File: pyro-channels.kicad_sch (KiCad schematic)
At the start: 22 parts, among them J2 Pyro Channels, J3 Screw Switches, Q2 AO3400A, Q3 AO3400A, Q5 AO3400A, Q6 AO3400A, Q7 AO3400A, Q8 AO3400A

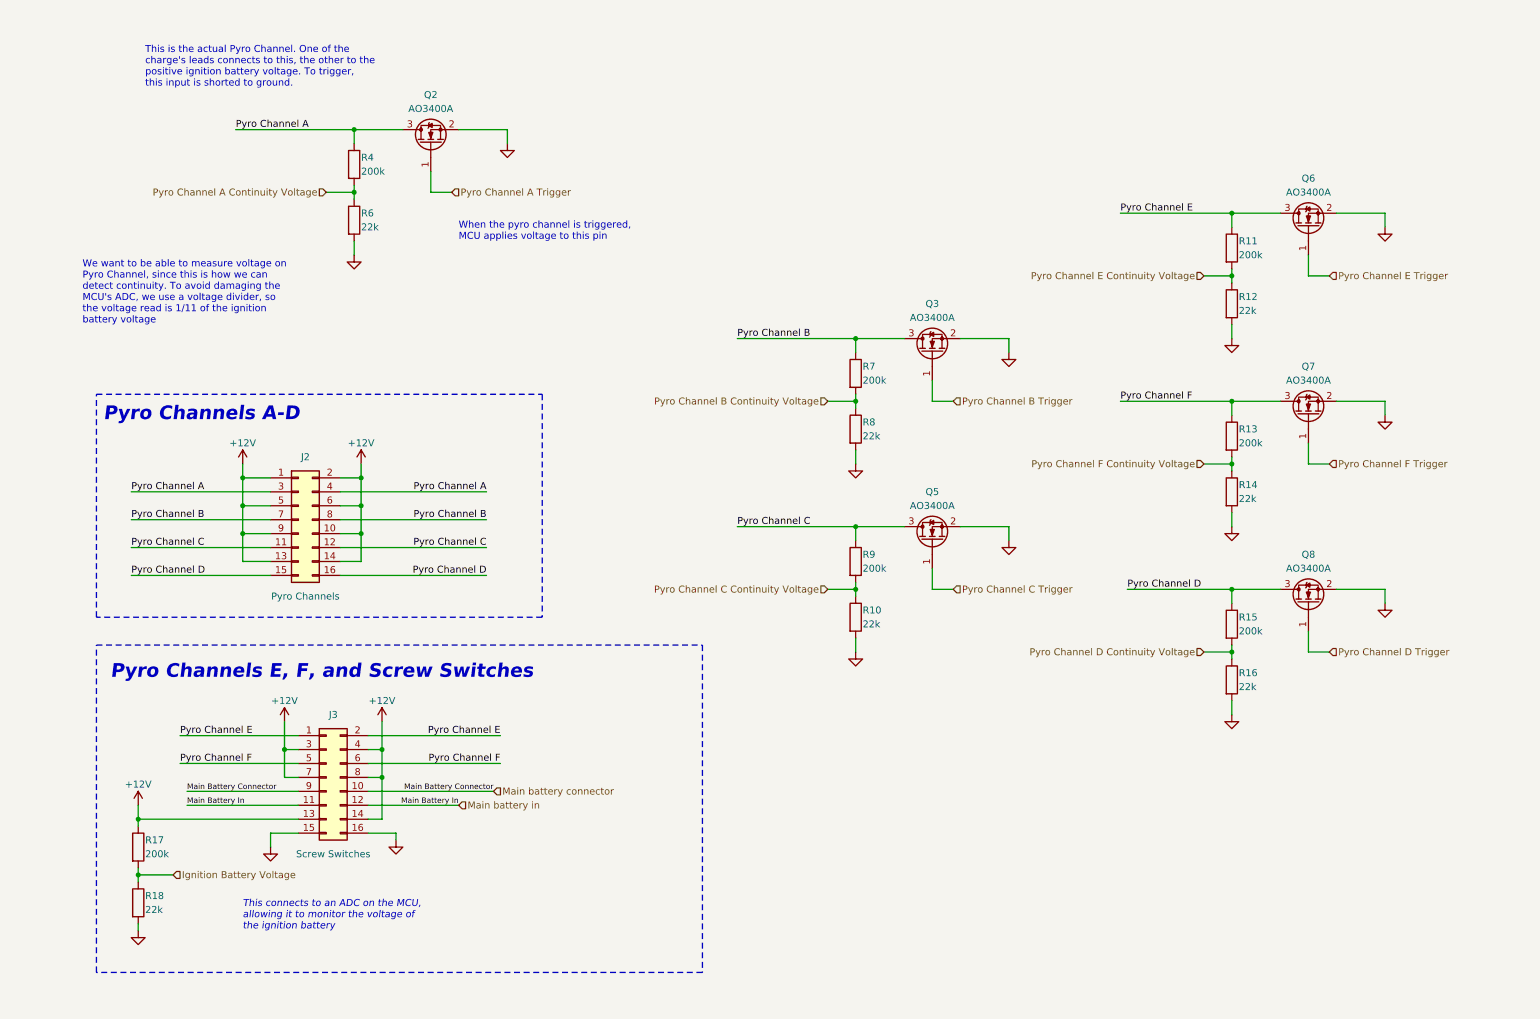
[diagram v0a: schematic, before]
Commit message: Finished updating the schematics
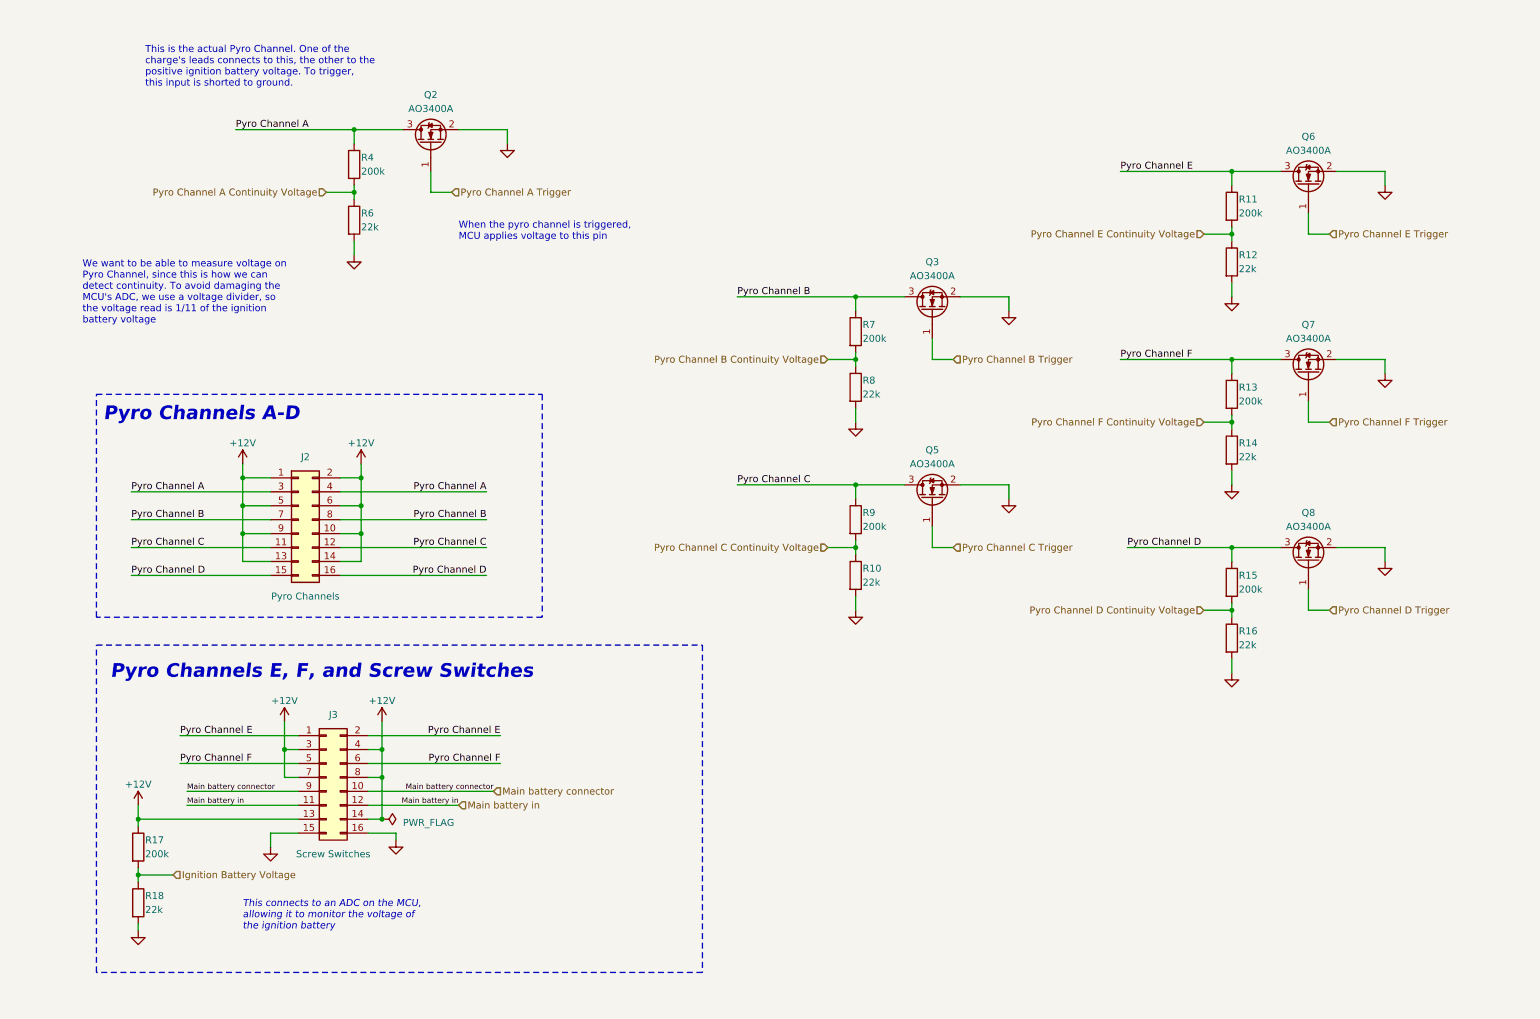
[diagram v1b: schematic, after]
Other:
- moved on the sheet: Q3, Q5, Q6, Q7, Q8, R10, R11, R12, R13, R14, R15, R16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

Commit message: Started doing layout for v1.1
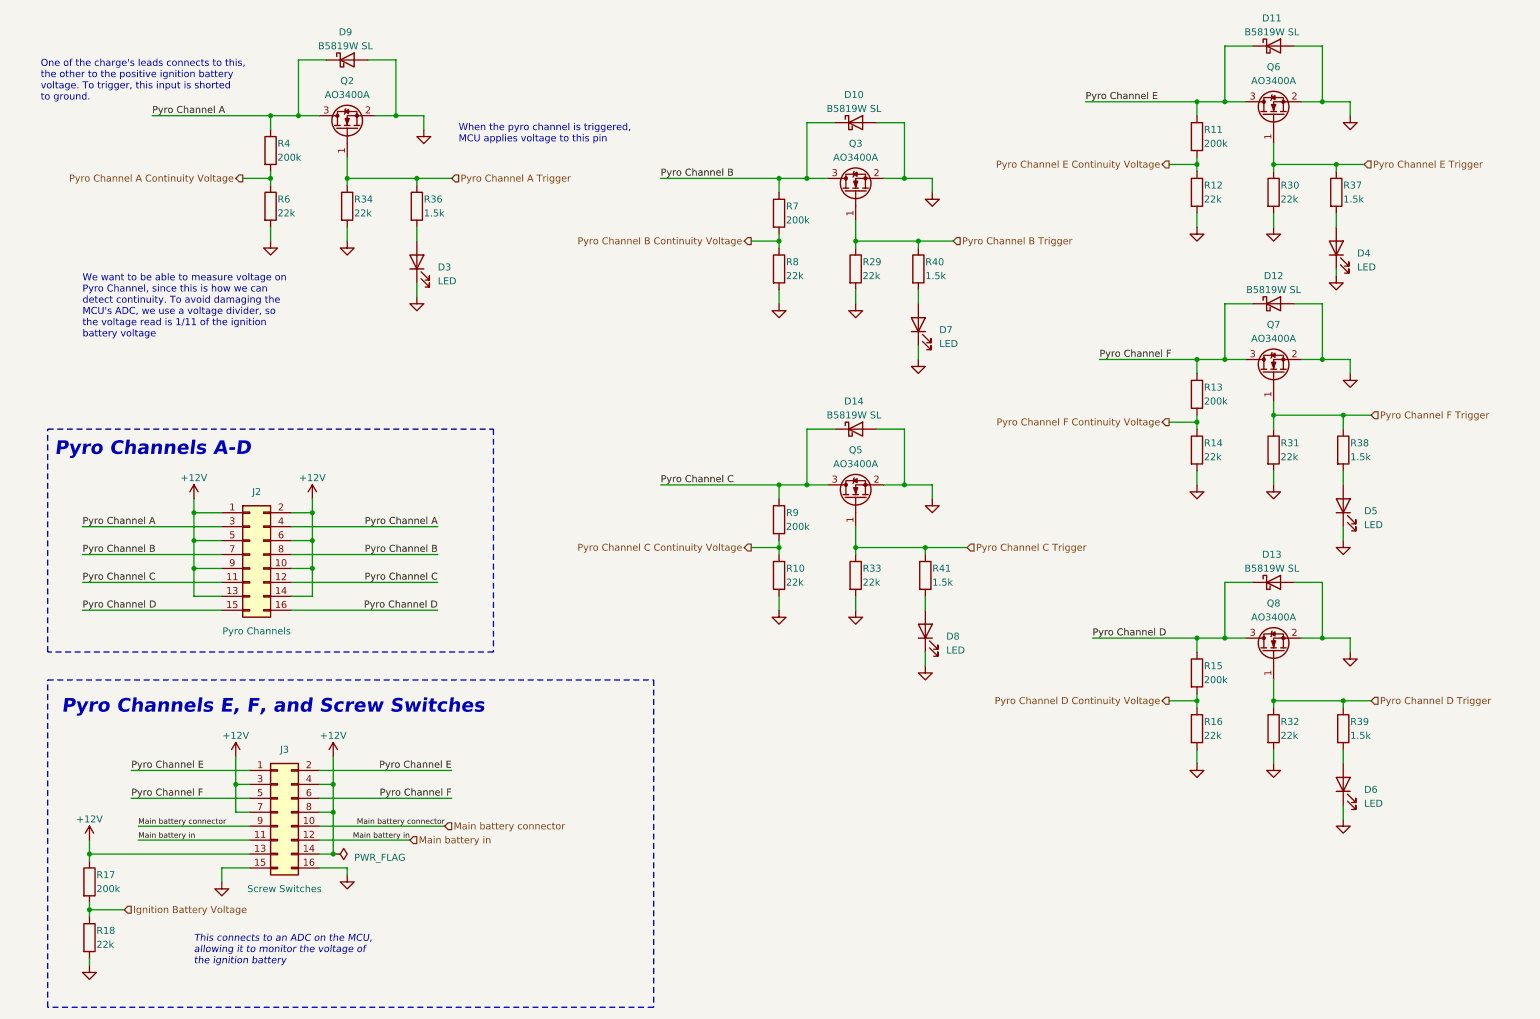
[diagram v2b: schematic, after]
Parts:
- added D10, D11, D12, D13, D14, D9: B5819W SL, Diode_SMD:D_SOD-123, symbol Device:D_Schottky
- added D3, D4, D5, D6, D7, D8: LED, LED_SMD:LED_0603_1608Metric_Pad1.05x0.95mm_HandSolder, symbol Device:LED
- added R29, R30, R31, R32, R33, R34: 22k, Resistor_SMD:R_0402_1005Metric, symbol Device:R
- added R36, R37, R38, R39, R40, R41: 1.5k, Resistor_SMD:R_0402_1005Metric, symbol Device:R
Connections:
- net GND: now also D10.2 (A), D11.2 (A), D12.2 (A), D13.2 (A), D14.2 (A), D3.1 (K), D4.1 (K), D5.1 (K), D6.1 (K), D7.1 (K), D8.1 (K), D9.2 (A), R29.2, R30.2, R31.2, R32.2, R33.2, R34.2
- net Pyro Channel A: now also D9.1 (K)
- net Pyro Channel A Trigger: now also R34.1, R36.1
- net Pyro Channel B: now also D10.1 (K)
- net Pyro Channel B Trigger: now also R29.1, R40.1
- net Pyro Channel C: now also D14.1 (K)
- net Pyro Channel C Trigger: now also R33.1, R41.1
- net Pyro Channel D: now also D13.1 (K)
- net Pyro Channel D Trigger: now also R32.1, R39.1
- net Pyro Channel E: now also D11.1 (K)
- net Pyro Channel E Trigger: now also R30.1, R37.1
- net Pyro Channel F: now also D12.1 (K)
- net Pyro Channel F Trigger: now also R31.1, R38.1
- new net: D5.2 (A), R38.2
- new net: D7.2 (A), R40.2
- new net: D3.2 (A), R36.2
- new net: D8.2 (A), R41.2
- new net: D6.2 (A), R39.2
- new net: D4.2 (A), R37.2
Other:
- note added: "One of the charge's leads connects to this, the other to the positive ignition battery voltage. To trigger, this input is shorted to ground."
- note removed: "This is the actual Pyro Channel. One of the charge's leads connects to this, the other to the positive ignition battery voltage. To trigger, this input is shorted to ground."
- moved on the sheet: J2, J3, Q2, Q3, Q5, Q6, Q7, Q8, R10, R11, R12, R13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
